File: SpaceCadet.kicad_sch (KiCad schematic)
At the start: 2 parts, among them U101 Pico

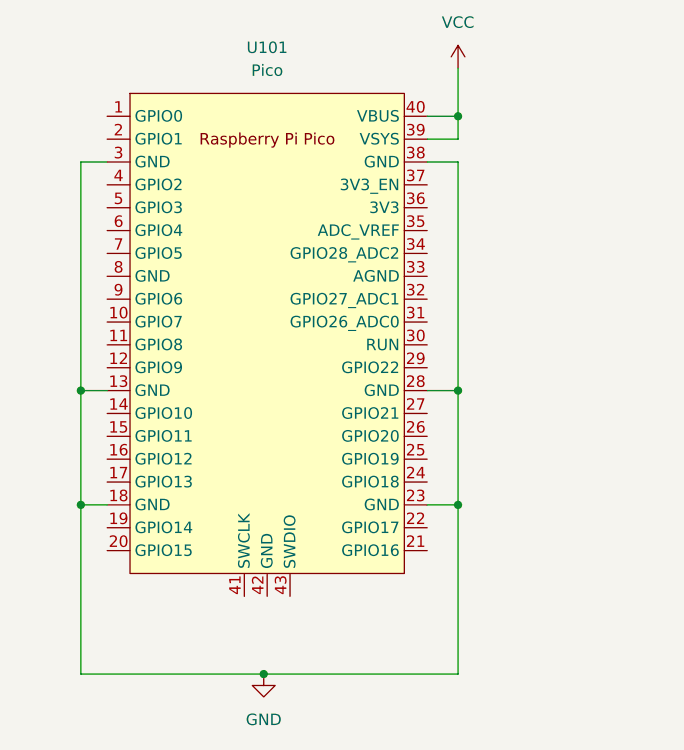
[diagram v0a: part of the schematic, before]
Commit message: wip: rpi pico on pcb
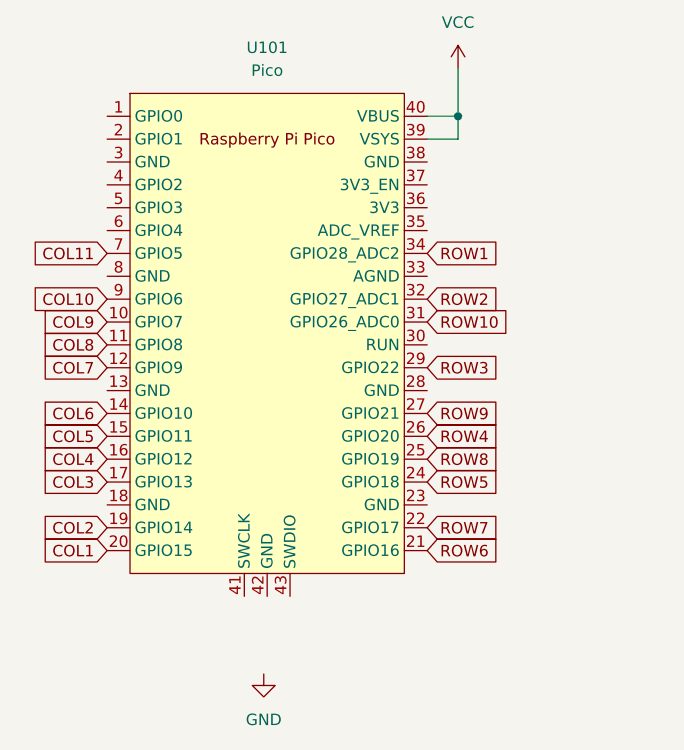
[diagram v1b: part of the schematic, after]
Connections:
- net GND: no longer U101.13 (GND), U101.18 (GND), U101.23 (GND), U101.28 (GND), U101.3 (GND), U101.38 (GND)
- net COL9: now reaches U101.10 (GPIO7)
- net COL8: now reaches U101.11 (GPIO8)
- net COL7: now reaches U101.12 (GPIO9)
- net COL6: now reaches U101.14 (GPIO10)
- net COL5: now reaches U101.15 (GPIO11)
- net COL4: now reaches U101.16 (GPIO12)
- net COL3: now reaches U101.17 (GPIO13)
- net COL2: now reaches U101.19 (GPIO14)
- net COL1: now reaches U101.20 (GPIO15)
- net ROW6: now reaches U101.21 (GPIO16)
- net ROW7: now reaches U101.22 (GPIO17)
- net ROW5: now reaches U101.24 (GPIO18)
- net ROW8: now reaches U101.25 (GPIO19)
- net ROW4: now reaches U101.26 (GPIO20)
- net ROW9: now reaches U101.27 (GPIO21)
- net ROW3: now reaches U101.29 (GPIO22)
- net ROW10: now reaches U101.31 (GPIO26_ADC0)
- net ROW2: now reaches U101.32 (GPIO27_ADC1)
- net ROW1: now reaches U101.34 (GPIO28_ADC2)
- net COL11: now reaches U101.7 (GPIO5)
- net COL10: now reaches U101.9 (GPIO6)

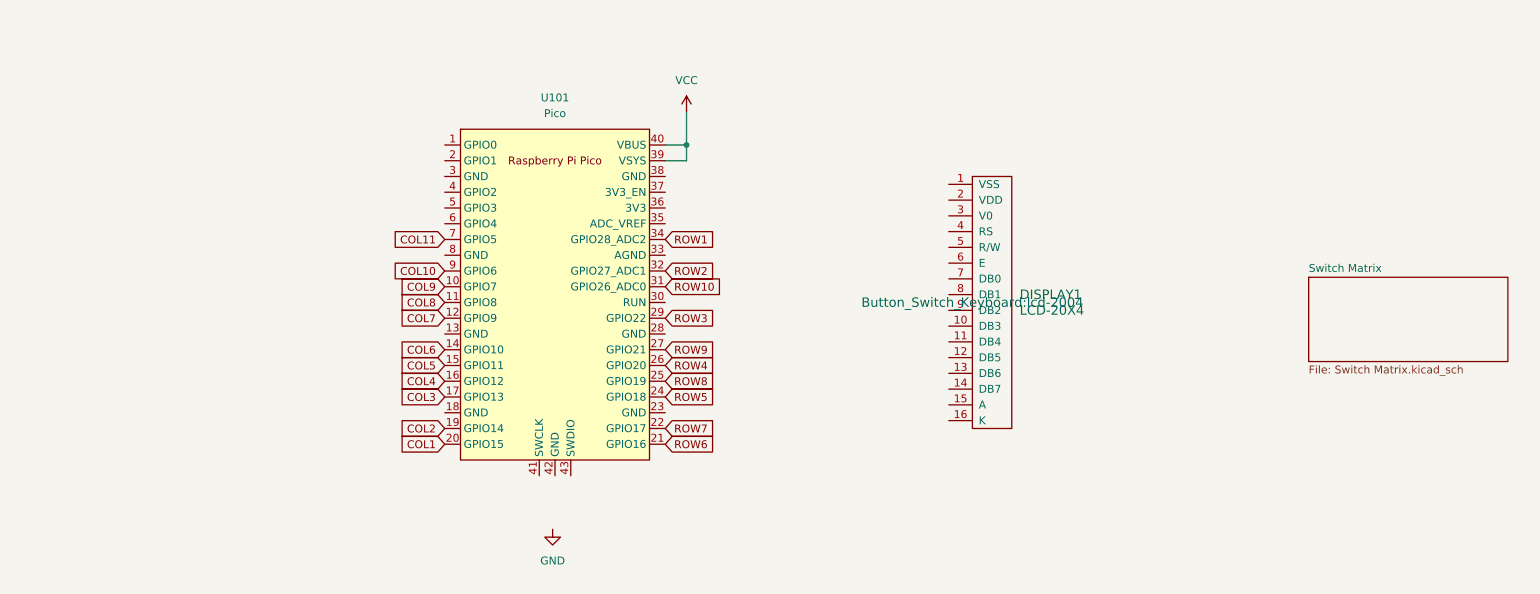
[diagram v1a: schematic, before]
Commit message: wip: pri fully connected with test points
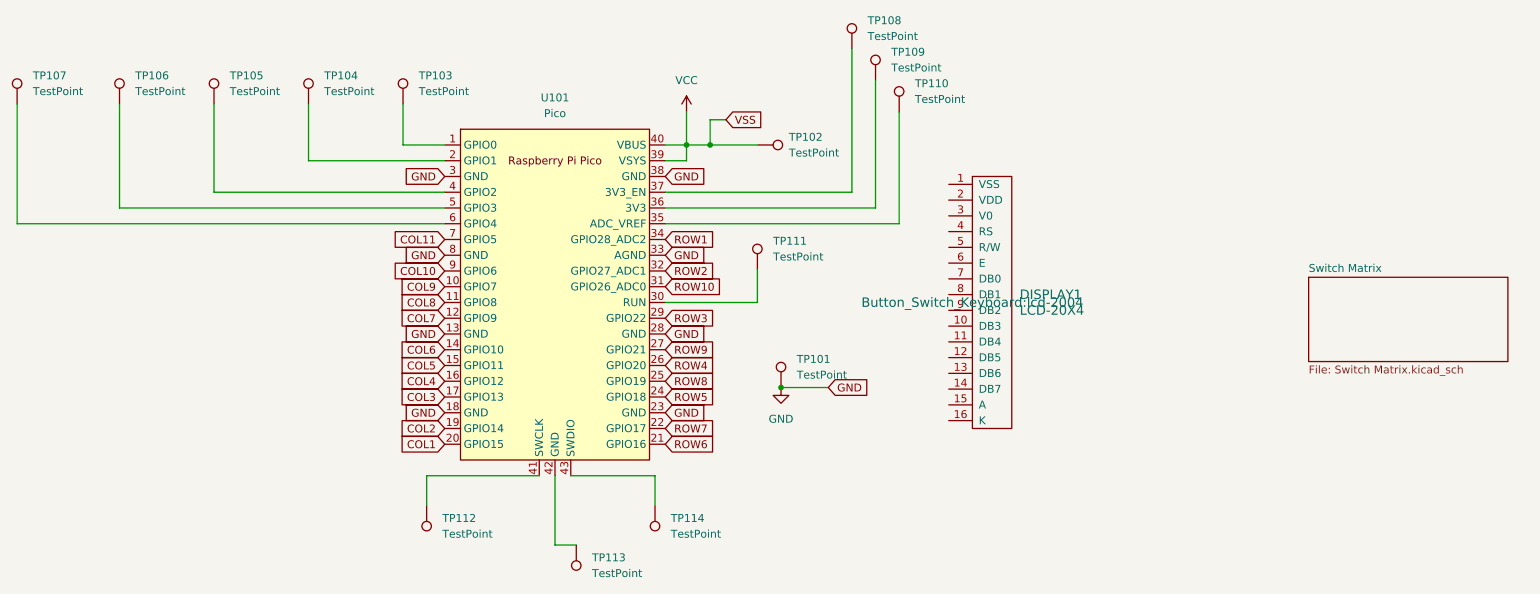
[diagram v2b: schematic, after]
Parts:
- added TP101, TP102, TP103, TP104, TP105, TP106, TP107, TP108, TP109, TP110, TP111, TP112, TP113, TP114: TestPoint, TestPoint:TestPoint_THTPad_2.0x2.0mm_Drill1.0mm, symbol Connector:TestPoint
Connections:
- net GND: now also U101.13 (GND), U101.18 (GND), U101.23 (GND), U101.28 (GND), U101.3 (GND), U101.33 (AGND), U101.38 (GND), U101.8 (GND), TP101.1
- net VCC: now also TP102.1
- net at U101.1 (GPIO0): now also TP103.1
- net at U101.2 (GPIO1): now also TP104.1
- net at U101.30 (RUN): now also TP111.1
- net at U101.35 (ADC_VREF): now also TP110.1
- net at U101.36 (3V3): now also TP109.1
- net at U101.37 (3V3_EN): now also TP108.1
- net at U101.4 (GPIO2): now also TP105.1
- net at U101.41 (SWCLK): now also TP112.1
- net at U101.42 (GND): now also TP113.1
- net at U101.43 (SWDIO): now also TP114.1
- net at U101.5 (GPIO3): now also TP106.1
- net at U101.6 (GPIO4): now also TP107.1
